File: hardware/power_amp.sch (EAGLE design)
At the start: 33 parts, among them X1 DEGSON_4, X2 DEGSON_3

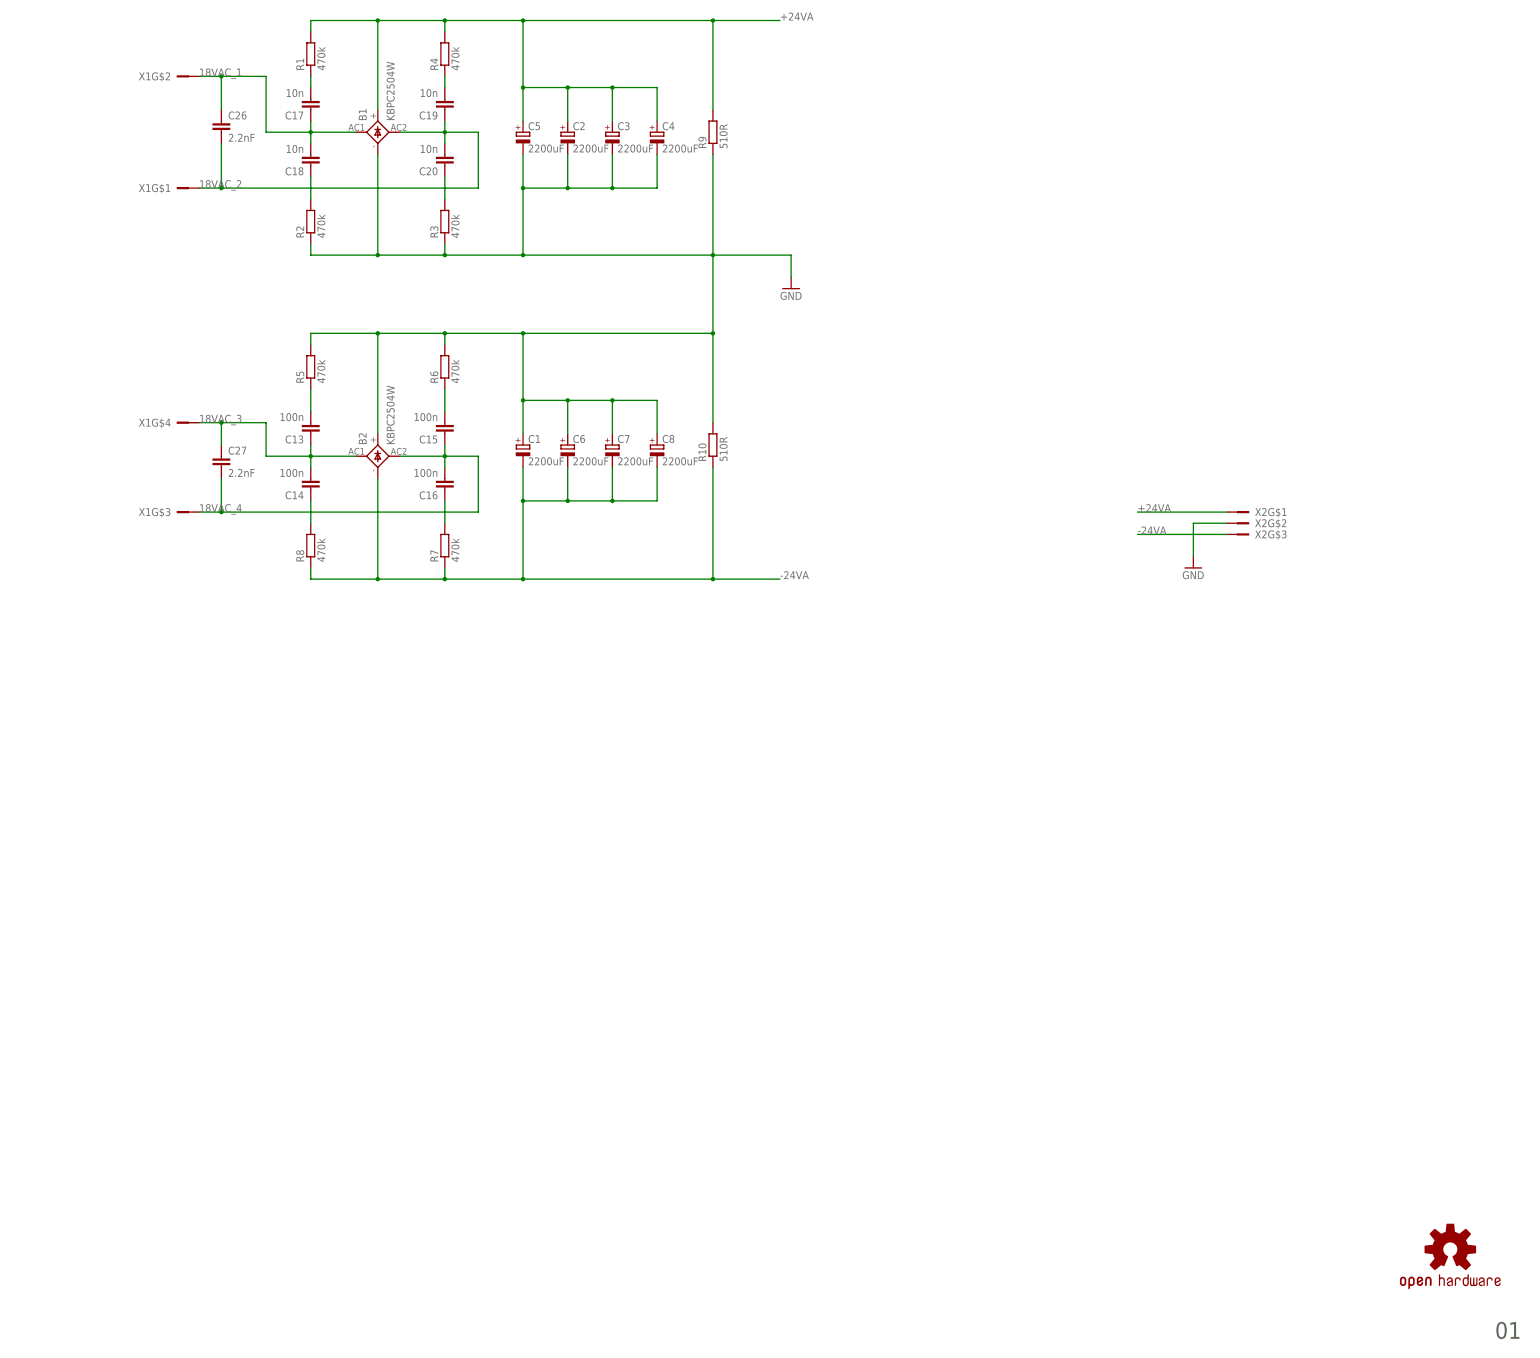
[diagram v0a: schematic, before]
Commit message: sent to manufacture
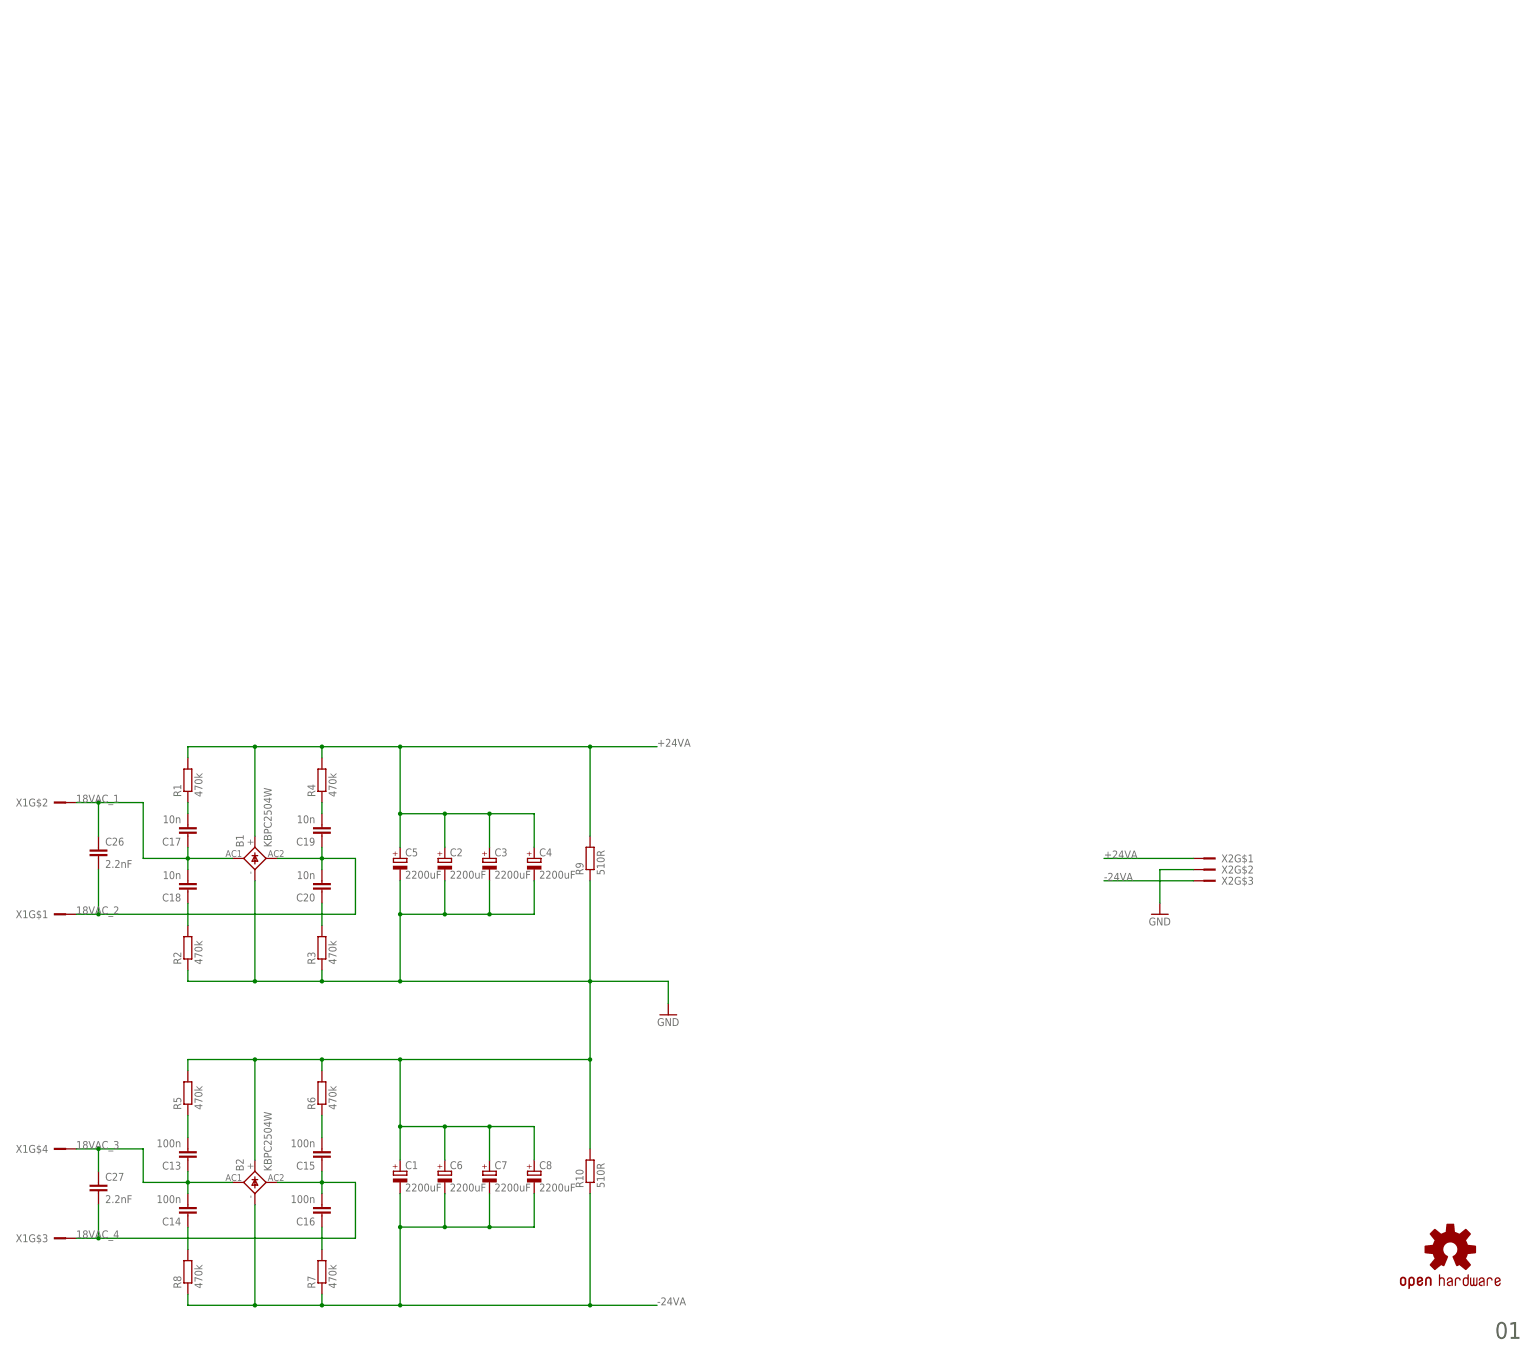
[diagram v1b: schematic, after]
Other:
- moved on the sheet: B1, B2, C1, C13, C14, C15, C16, C17, C18, C19, C2, C20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
